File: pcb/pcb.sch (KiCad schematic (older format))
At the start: 16 parts, among them J1 VIN VBAT, J2 Conn_01x04, J3 AudioJack3, J4 Conn_01x04, J5 HX711, J6 Conn_01x04, J7 Conn_01x04, U1 LM386, U2 WSSFM10R1AT

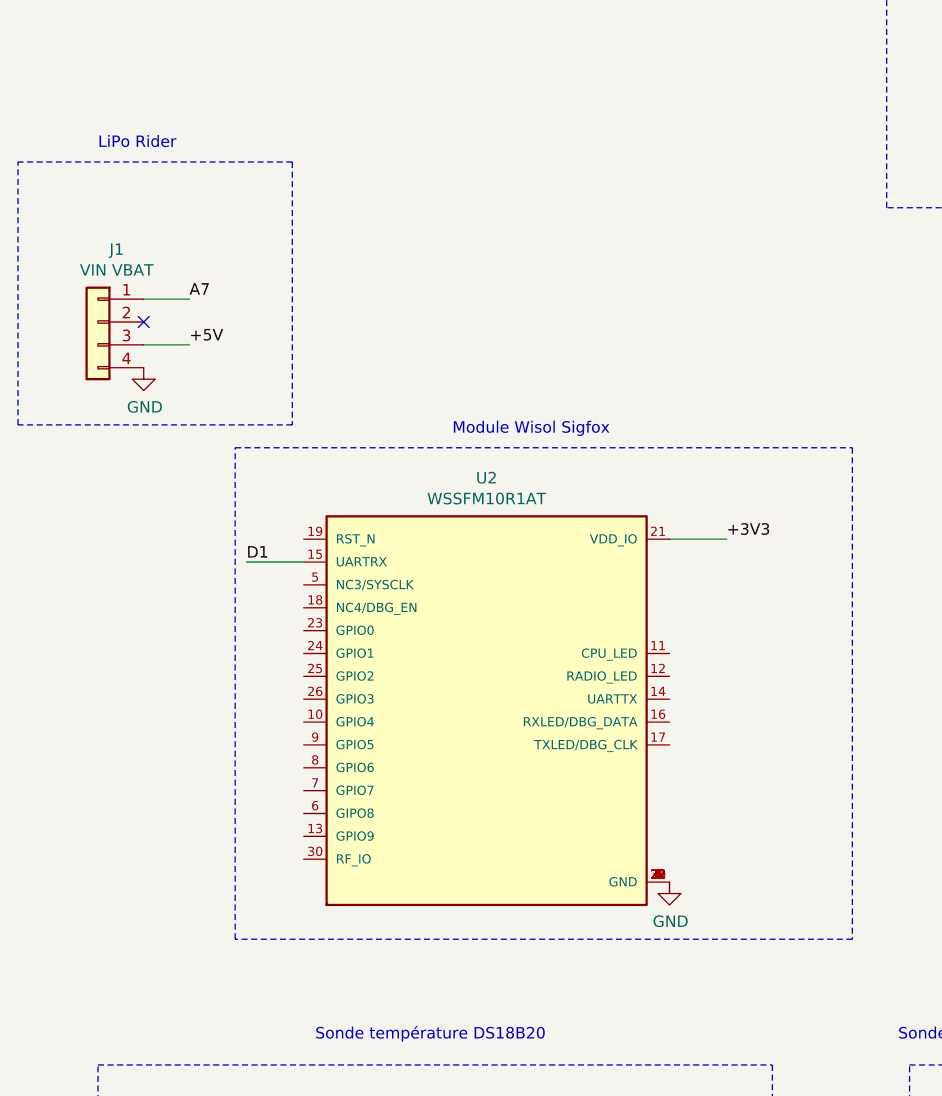
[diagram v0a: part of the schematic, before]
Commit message: Finalisation PCB
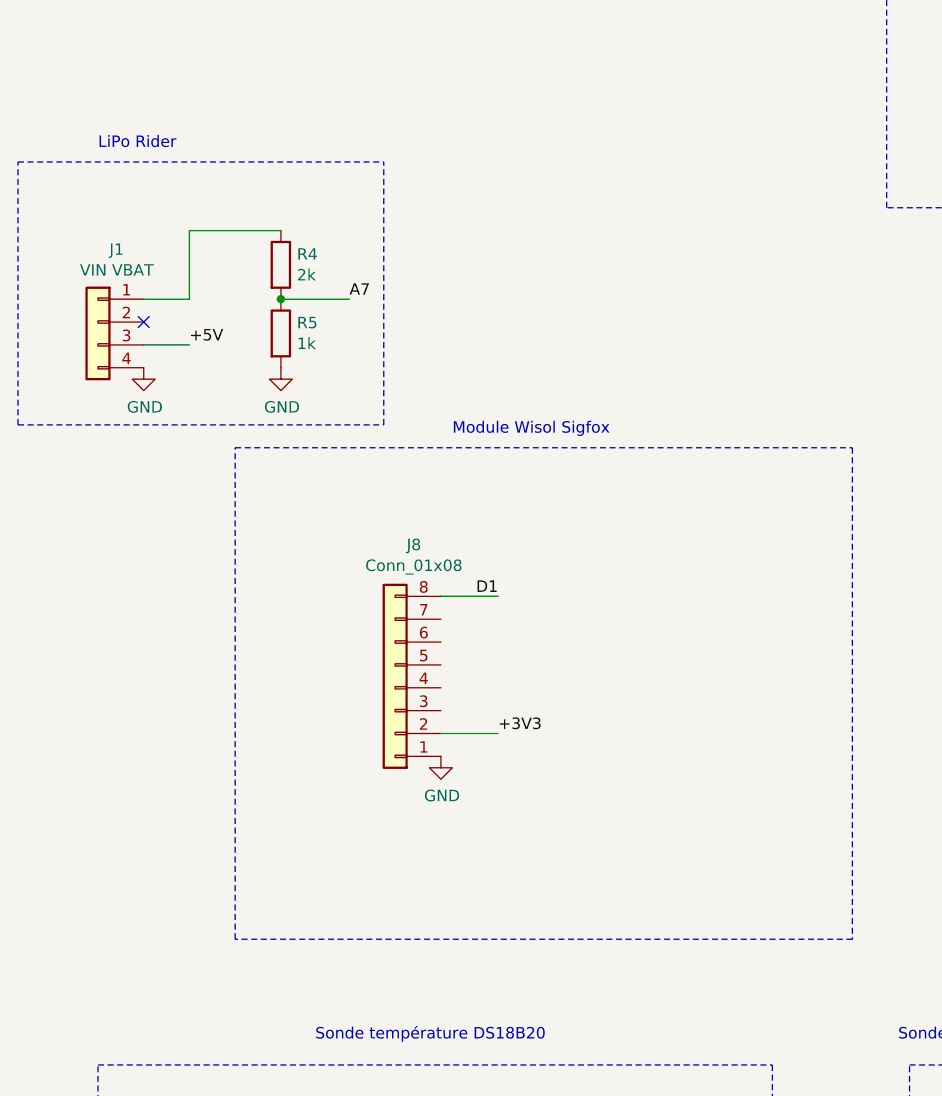
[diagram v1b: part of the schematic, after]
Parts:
- removed U2: WSSFM10R1AT, WSSFM10R1AT:XCVR_WSSFM10R1AT, symbol WSSFM10R1AT:WSSFM10R1AT
- added J8: Conn_01x08, Connector_PinHeader_2.00mm:PinHeader_1x08_P2.00mm_Vertical, symbol Connector_Generic:Conn_01x08
- added R4: 2k, Resistor_THT:R_Axial_DIN0204_L3.6mm_D1.6mm_P5.08mm_Vertical, symbol Device:R
- added R5: 1k, Resistor_THT:R_Axial_DIN0204_L3.6mm_D1.6mm_P5.08mm_Vertical, symbol Device:R
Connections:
- net +3V3: now also J8.2 (Pin_2)
- net A7: now also R4.2, R5.1; no longer J1.1 (Pin_1)
- net D1: now also J8.8 (Pin_8)
- net GND: now also J8.1 (Pin_1), R5.2
- new net: J1.1 (Pin_1), R4.1
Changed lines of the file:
@@
 Text Label 6650 3500 0    50   ~ 0
-A7
-Text Label 1400 2250 0    50   ~ 0
 A7
 $Comp
@@
 Text Label 5050 3600 0    50   ~ 0
 D3
-Wire Notes Line
-	1850 1650 1850 2800
-Wire Notes Line
-	1850 2800 650  2800
 Wire Notes Line
 	650  2800 650  1650
@@
 $EndComp
 NoConn ~ 1200 2350
-Wire Notes Line
-	1850 1650 650  1650
 $Comp
 L Device:R R1
@@
 $EndComp
 $Comp
-L WSSFM10R1AT:WSSFM10R1AT U2
-U 1 1 5FB95228
-P 2700 3900
-F 0 "U2" H 2700 4767 50  0000 C CNN
-F 1 "WSSFM10R1AT" H 2700 4676 50  0000 C CNN
-F 2 "WSSFM10R1AT:XCVR_WSSFM10R1AT" H 2700 3900 50  0001 L BNN
-F 3 "" H 2700 3900 50  0001 L BNN
-F 4 "WISOL" H 2700 3900 50  0001 L BNN "MANUFACTURER"
-	1    2700 3900
-	1    0    0    -1
-$EndComp
-$Comp
 L power:GND #PWR0117
 U 1 1 5FB961B3
-P 3500 4800
-F 0 "#PWR0117" H 3500 4550 50  0001 C CNN
-F 1 "GND" H 3505 4627 50  0000 C CNN
-F 2 "" H 3500 4800 50  0001 C CNN
-F 3 "" H 3500 4800 50  0001 C CNN
-	1    3500 4800
-	1    0    0    -1
-$EndComp
-Wire Wire Line
-	3500 3300 3750 3300
-Text Label 3750 3300 0    50   ~ 0
+P 2500 4250
+F 0 "#PWR0117" H 2500 4000 50  0001 C CNN
+F 1 "GND" H 2505 4077 50  0000 C CNN
+F 2 "" H 2500 4250 50  0001 C CNN
+F 3 "" H 2500 4250 50  0001 C CNN
+	1    2500 4250
+	1    0    0    -1
+$EndComp
+Wire Wire Line
+	2500 4150 2750 4150
+Text Label 2750 4150 0    50   ~ 0
 +3V3
 Wire Wire Line
@@
 D1
 Wire Wire Line
-	1900 3400 1650 3400
-Text Label 1650 3400 0    50   ~ 0
+	2500 3550 2750 3550
+Text Label 2750 3550 2    50   ~ 0
 D1
 Wire Notes Line
@@
 Text Notes 2550 2850 0    50   ~ 0
 Module Wisol Sigfox
+$Comp
+L Device:R R4
+U 1 1 5FBBD368
+P 1800 2100
+F 0 "R4" H 1870 2146 50  0000 L CNN
+F 1 "2k" H 1870 2055 50  0000 L CNN
+F 2 "Resistor_THT:R_Axial_DIN0204_L3.6mm_D1.6mm_P5.08mm_Vertical" V 1730 2100 50  0001 C CNN
+F 3 "~" H 1800 2100 50  0001 C CNN
+	1    1800 2100
+	1    0    0    -1
+$EndComp
+$Comp
+L Device:R R5
+U 1 1 5FBBD807
+P 1800 2400
+F 0 "R5" H 1870 2446 50  0000 L CNN
+F 1 "1k" H 1870 2355 50  0000 L CNN
+F 2 "Resistor_THT:R_Axial_DIN0204_L3.6mm_D1.6mm_P5.08mm_Vertical" V 1730 2400 50  0001 C CNN
+F 3 "~" H 1800 2400 50  0001 C CNN
+	1    1800 2400
+	1    0    0    -1
+$EndComp
+$Comp
+L power:GND #PWR0118
+U 1 1 5FBBDDB8
+P 1800 2550
+F 0 "#PWR0118" H 1800 2300 50  0001 C CNN
+F 1 "GND" H 1805 2377 50  0000 C CNN
+F 2 "" H 1800 2550 50  0001 C CNN
+F 3 "" H 1800 2550 50  0001 C CNN
+	1    1800 2550
+	1    0    0    -1
+$EndComp
+Wire Wire Line
+	1400 2250 1400 1950
+Wire Wire Line
+	1400 1950 1800 1950
+Wire Wire Line
+	1800 2250 2100 2250
+Connection ~ 1800 2250
+Text Label 2100 2250 0    50   ~ 0
+A7
+Wire Notes Line
+	2250 2800 2250 1650
+Wire Notes Line
+	650  2800 2250 2800
+Wire Notes Line
+	650  1650 2250 1650
+$Comp
+L Connector_Generic:Conn_01x08 J8
+U 1 1 5FBC63C9
+P 2300 3950
+F 0 "J8" H 2218 3325 50  0000 C CNN
+F 1 "Conn_01x08" H 2218 3416 50  0000 C CNN
+F 2 "Connector_PinHeader_2.00mm:PinHeader_1x08_P2.00mm_Vertical" H 2300 3950 50  0001 C CNN
+F 3 "~" H 2300 3950 50  0001 C CNN
+	1    2300 3950
+	-1   0    0    1
+$EndComp
 $EndSCHEMATC
